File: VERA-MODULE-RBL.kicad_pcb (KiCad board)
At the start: 4 copper layers, 143 x 162.5 mm, 175 parts, among them J1 CONN_SMD_02x08_Odd_Even_2.54mm, J2 ICD15S13E4GX00LF, J3 CONN_DM3AT-SF-PEJM5, J4 DX07S016JA1R1500, J5 PJ-002AH-SMT-TR, Q1 MOSFET-BSS138-SOT-23, Q2 MOSFET-BSS138-SOT-23, Q3 BC817,SOT-23, Q4 BC817,SOT-23, Q5 MOSFET-BSS138-SOT-23, SW1 SPST2P, SW2 SPST_SWITCH_SMD_4P,4.1x5.4mm, U1 TXS0108EPW, U10 W25Q16JVSNIQ, U11 WM8524CGEDT, U12 USBCH340T, U13 AMS1117-3.3, U14 AMS1117-2.5, U15 L7805, U16 TXS0108EPW, U17 MAX40200AUK, U2 ICE40UP5K-SG48ITR, U3 TXS0108EPW, U4 TXS0108EPW, U5 IC74HC00, U6 TXS0108EPW, U7 ESP32-PICO-D4, U8 74CBTLV3126PW,118, U9 IC74HC00, X1 SG-5032CAN, Y1 12MHzC

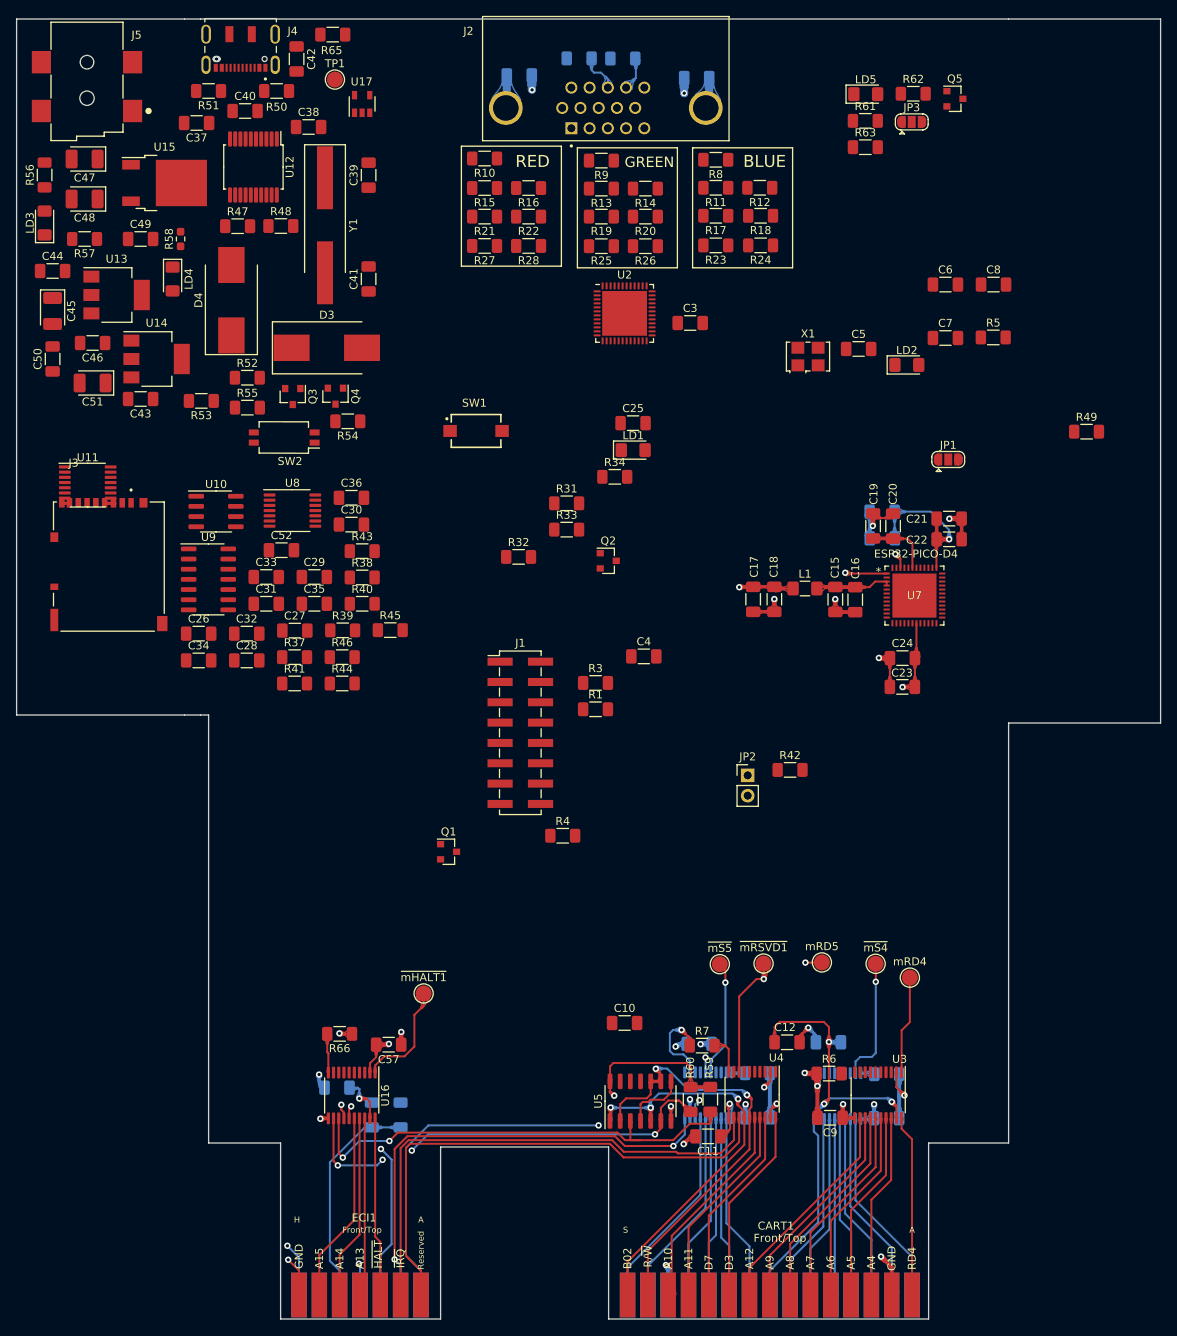
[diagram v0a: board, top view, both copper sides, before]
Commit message: Updated
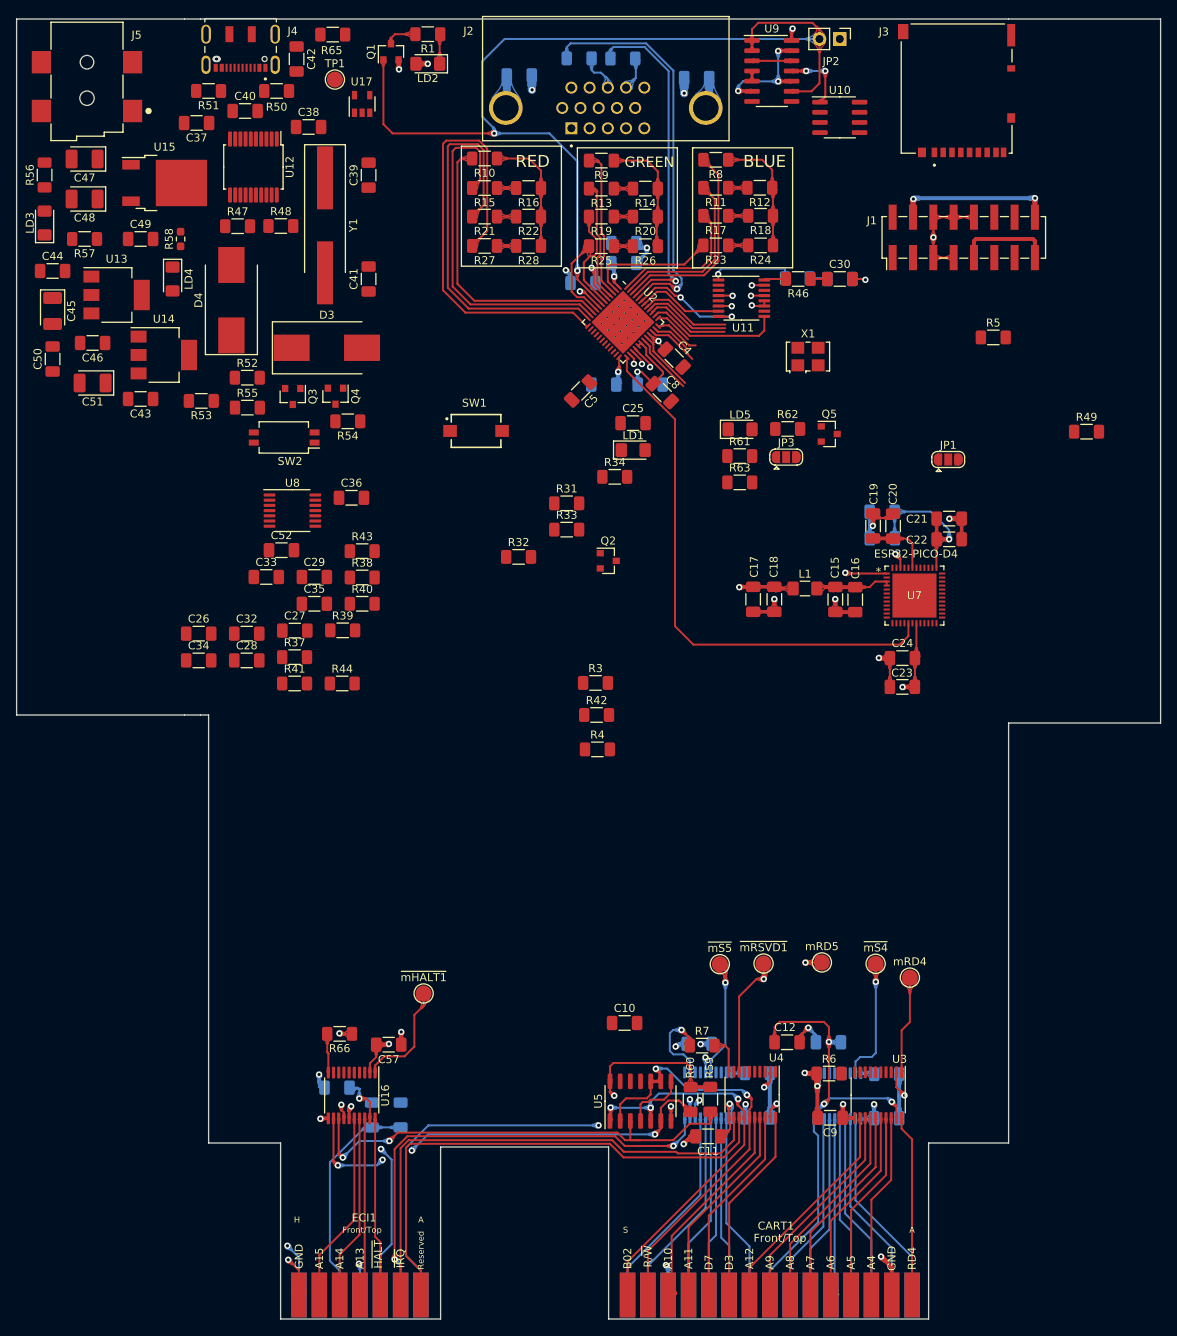
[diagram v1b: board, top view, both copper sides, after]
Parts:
- added C59: 1uF, Capacitor_SMD:C_1206_3216Metric_Pad1.33x1.80mm_HandSolder, B.Cu at (205.9, 93.2)
- added C60: 1uF, Capacitor_SMD:C_1206_3216Metric_Pad1.33x1.80mm_HandSolder, B.Cu at (211.7, 93.2)
- C3, C31, C6, C7, R45: moved to B.Cu
- U14: value AMS1117-2.5 -> AMS1117-1.5
- U2: footprint Package_DFN_QFN:QFN-48-1EP_7x7mm_P0.5mm_EP5.6x5.6mm -> RetroBitLab:QFN-48-1EP_7x7mm_P0.5mm_EP5.6x5.6mm
- moved J3 121.6 mm to (250.0, 56.2), turned to 180 degrees
- moved Q1 100.3 mm to (179.3, 51.6), turned to 90 degrees
- moved U9 94.9 mm to (226.9, 54.0)
- moved JP2 92.8 mm to (235.4, 50.0), turned to 270 degrees
- moved U10 92.2 mm to (235.4, 59.8)
- moved R1 87.0 mm to (183.9, 49.4), turned to 180 degrees
- moved U11 85.0 mm to (223.1, 82.4)
- moved J1 83.1 mm to (250.9, 74.8), turned to 90 degrees
- moved C31 82.4 mm to (235.4, 80.0)
- moved R46 74.1 mm to (230.2, 80.0), turned to 180 degrees
- moved LD2 70.7 mm to (183.9, 53.1), turned to 180 degrees
- moved C30 68.3 mm to (235.4, 80.0)
- moved R45 67.3 mm to (230.1, 79.9), turned to 180 degrees
- moved C7 45.8 mm to (203.3, 80.5), turned to 180 degrees
- moved JP3 44.7 mm to (228.7, 102.3)
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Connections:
- C3 pad 2: +3V3 -> 3V3
- C4 pad 1: +3V3 -> 3V3
- C43 pad 1: 2V5 -> 1V5
- C5 pad 1: +3V3 -> 3V3
- C51 pad 1: 2V5 -> 1V5
- C6 pad 1: +3V3 -> 3V3
- C7 pad 1: Net-(C7-Pad1) -> 1V5
- C8 pad 1: Net-(C7-Pad1) -> 1V5
- J1 pad 11: Net-(J1-Pad11) -> AUDIOL
- J1 pad 12: Net-(J1-Pad12) -> AUDIOR
- J1 pad 15: Net-(J1-Pad15) -> 5V
- J1 pad 16: Net-(J1-Pad16) -> 3V3
- J1 pad 4: Net-(J1-Pad4) -> 3V3
- J1 pad 9: +5V -> 5V
- R5 pad 1: +3V3 -> 3V3
- U14 pad 2: 2V5 -> 1V5
- U2 pad 1: +3V3 -> 3V3
- U2 pad 22: +3V3 -> 3V3
- U2 pad 24: 2V5 -> 3V3
- U2 pad 29: Net-(C7-Pad1) -> 1V5
- U2 pad 30: Net-(C7-Pad1) -> 1V5
- U2 pad 33: +3V3 -> 3V3
- U2 pad 44: /VeraModule/VGA_VSYNC -> /VeraModule/VGA_HSYNC
- U2 pad 45: /VeraModule/VGA_HSYNC -> /VeraModule/VGA_VSYNC
- U2 pad 5: Net-(C7-Pad1) -> 1V5
- X1 pad 4: +3V3 -> 3V3
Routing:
- net FPGA_CDONE: track 0.00 -> 128.7 mm, vias 0 -> 2
- net mD2: track 0.00 -> 68.3 mm
- net /VeraModule/VGA_R3: track 0.00 -> 57.3 mm
- net /VeraModule/VGA_R2: track 0.00 -> 50.6 mm
- net /VeraModule/VGA_HSYNC: track 0.00 -> 50.2 mm, vias 0 -> 1
- net /VeraModule/VGA_R1: track 0.00 -> 44.5 mm
- net /VeraModule/VGA_VSYNC: track 0.00 -> 42.3 mm, vias 0 -> 1
- net 3V3: track 51.9 -> 88.7 mm, vias 5 -> 14
- net /VeraModule/VGA_R0: track 0.00 -> 35.8 mm
- net GND: track 67.0 -> 93.6 mm, vias 19 -> 26
- net /VeraModule/VGA_B0: track 0.00 -> 25.8 mm
- net /VeraModule/VGA_B1: track 0.00 -> 21.8 mm
- net /VeraModule/VGA_G0: track 0.00 -> 18.7 mm
- net 1V5: track 0.00 -> 18.3 mm, vias 0 -> 2
- net /VeraModule/VGA_B2: track 0.00 -> 17.7 mm
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- removed copper zone on POWER, net 3V3
- removed copper zone on GND, net GND
